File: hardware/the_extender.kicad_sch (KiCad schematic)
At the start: 122 parts, among them J0 TYPE-C 24P QT 143, J1 TYPE-C-31-M-16, J2 U231-091N-3BLRC11, J3 PJ-327D-5A, J4 PJ-327D-5A, J5 AF 10.0 HC6.3, Q4 SSM3J332R,LF, Q6 SSM3J332R,LF, U0 RT6150BGQW, U1 IP5306-I2C, U2 RP2040, U3 W25Q32JVSS, U4 FUSB302BMPX, U5 USB2514B_Bi, U6 HS-100B, Y1 ABLS-12.000MHZ-20-B-3-H-T

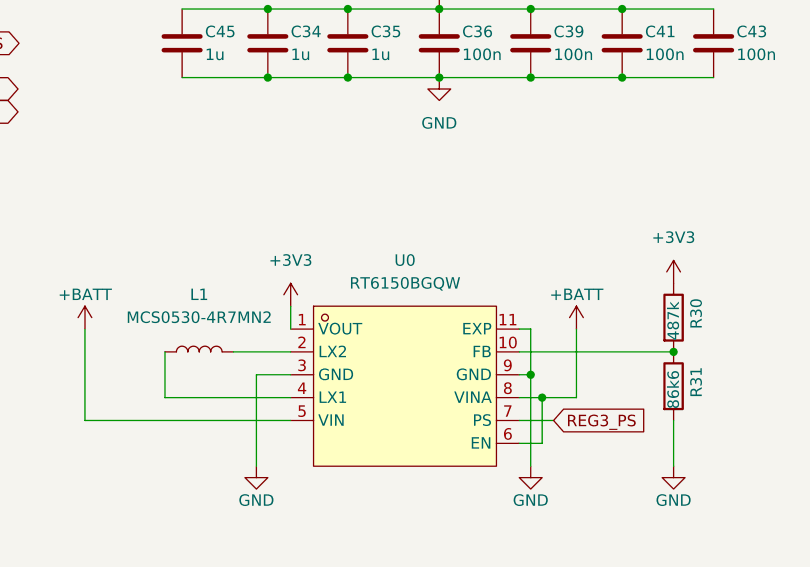
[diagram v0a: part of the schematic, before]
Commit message: switch 3v3 footprint, fixup stuff
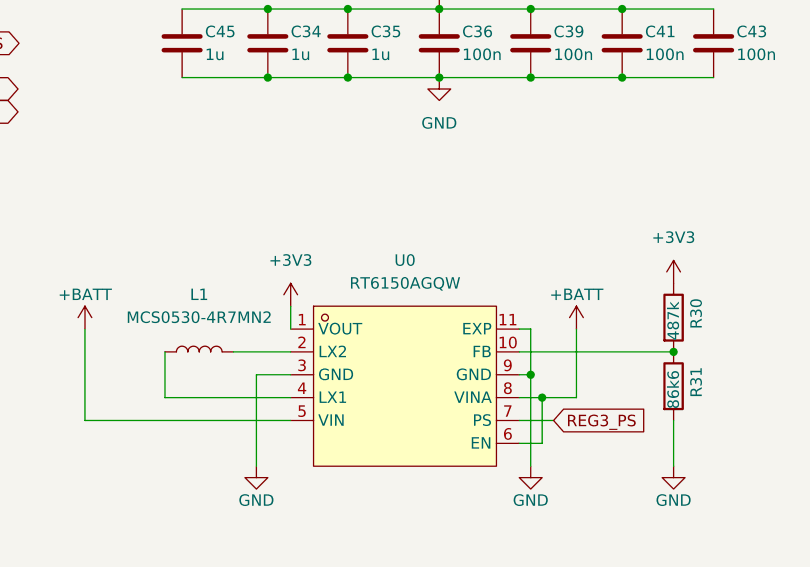
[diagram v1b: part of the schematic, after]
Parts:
- U0: value RT6150BGQW -> RT6150AGQW; footprint Package_SON:WSON-10-1EP_2.5x2.5mm_P0.5mm_EP1.2x2mm -> Package_DFN_QFN:WDFN-10-1EP_3x3mm_P0.5mm_EP1.8x2.5mm
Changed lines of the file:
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@@
       (effects (font (size 1.27 1.27)))
     )
-    (property "Value" "RT6150BGQW" (at 354.33 215.9 0)
+    (property "Value" "RT6150AGQW" (at 354.33 215.9 0)
       (effects (font (size 1.27 1.27)))
     )
-    (property "Footprint" "Package_SON:WSON-10-1EP_2.5x2.5mm_P0.5mm_EP1.2x2mm" (at 354.33 241.3 0)
+    (property "Footprint" "Package_DFN_QFN:WDFN-10-1EP_3x3mm_P0.5mm_EP1.8x2.5mm" (at 354.33 241.3 0)
       (effects (font (size 1.27 1.27)) hide)
     )
